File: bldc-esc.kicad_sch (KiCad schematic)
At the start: 0 parts

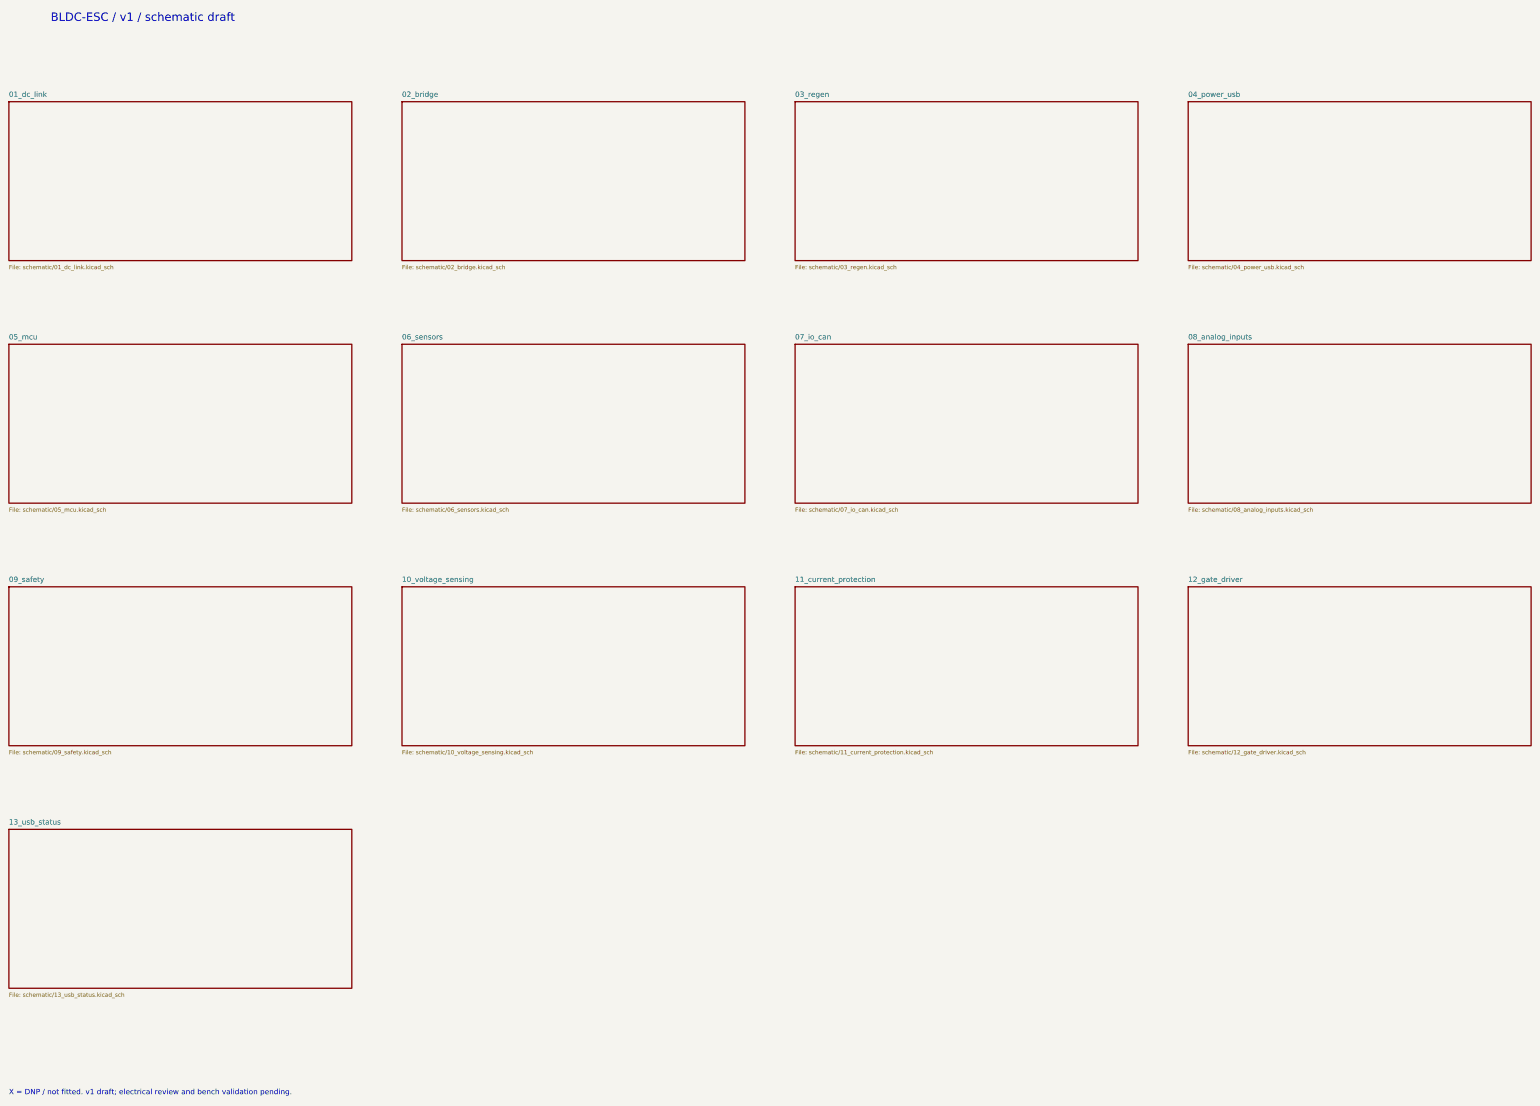
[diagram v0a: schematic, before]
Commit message: devlog 03
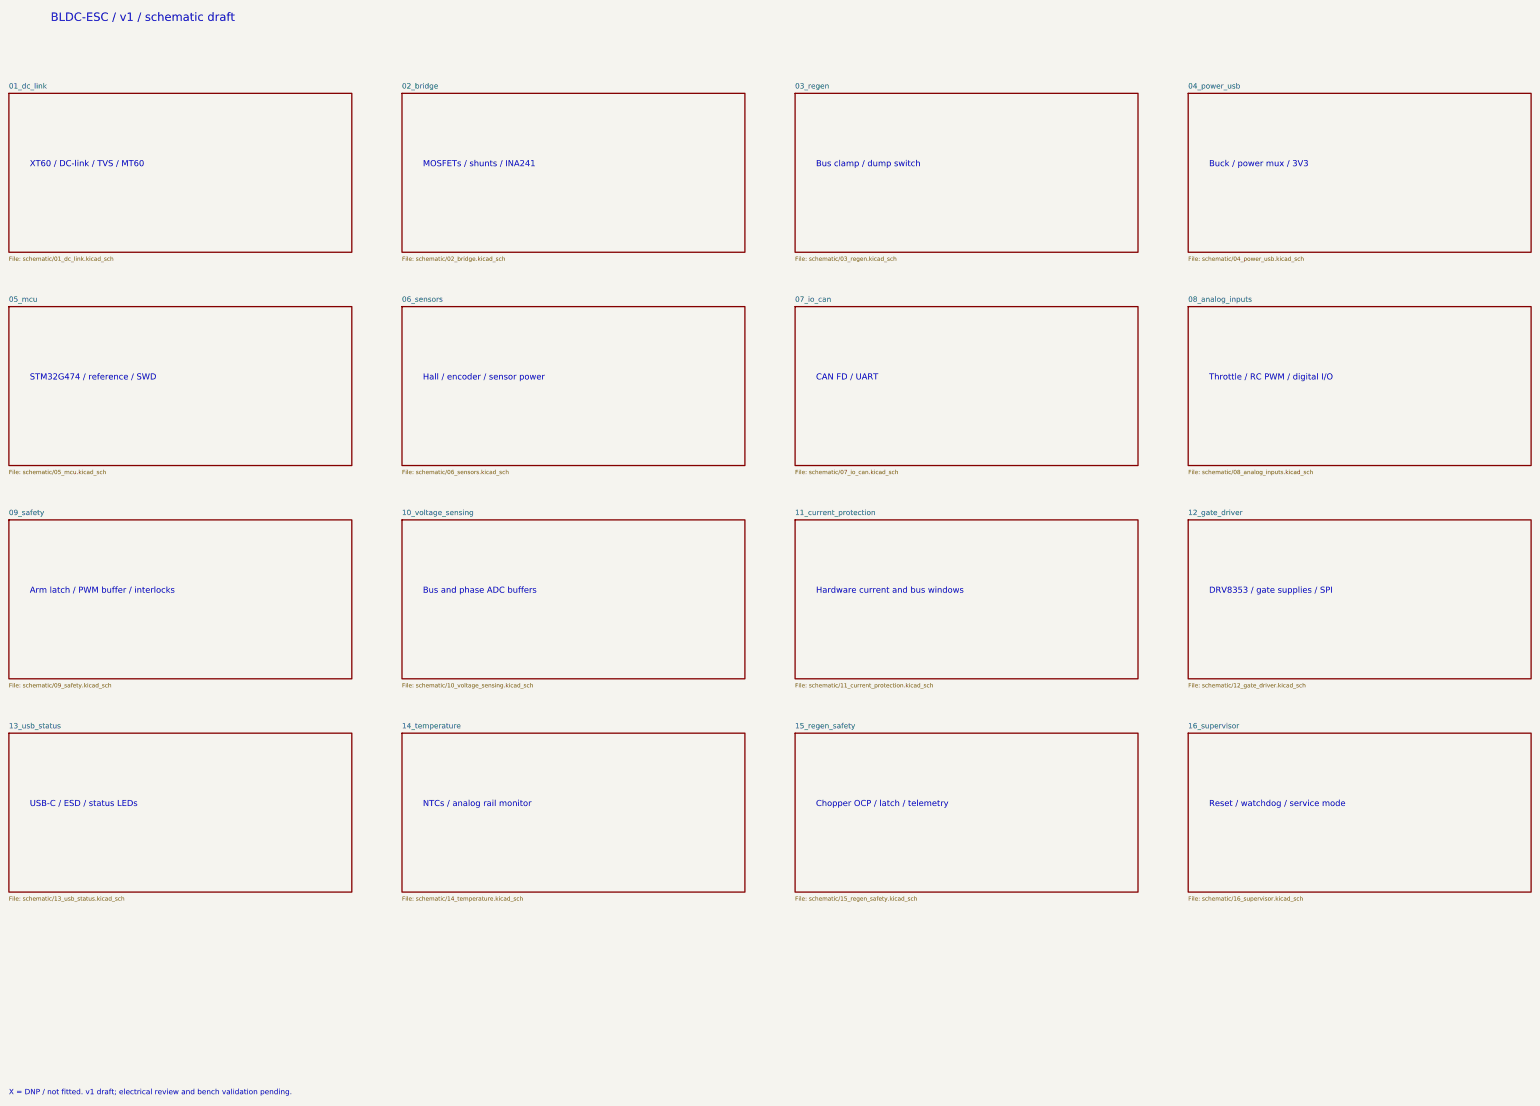
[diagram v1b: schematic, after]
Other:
- added sheet 14_temperature (schematic/14_temperature.kicad_sch)
- added sheet 15_regen_safety (schematic/15_regen_safety.kicad_sch)
- added sheet 16_supervisor (schematic/16_supervisor.kicad_sch)
- note added: "Arm latch / PWM buffer / interlocks"
- note added: "Buck / power mux / 3V3"
- note added: "Bus and phase ADC buffers"
- note added: "Bus clamp / dump switch"
- note added: "CAN FD / UART"
- note added: "Chopper OCP / latch / telemetry"
- note added: "DRV8353 / gate supplies / SPI"
- note added: "Hall / encoder / sensor power"
- note added: "Hardware current and bus windows"
- note added: "MOSFETs / shunts / INA241"
- note added: "NTCs / analog rail monitor"
- note added: "Reset / watchdog / service mode"
- note added: "STM32G474 / reference / SWD"
- note added: "Throttle / RC PWM / digital I/O"
- note added: "USB-C / ESD / status LEDs"
- note added: "XT60 / DC-link / TVS / MT60"
